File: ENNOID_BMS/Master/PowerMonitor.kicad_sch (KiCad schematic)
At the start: 103 parts, among them J15 Charge +, U1 AMC1301 or AMC1302, U10 SN6501DBV, U12 AMC1301, U13 AMC1301, U15A OPA2197IDR, U15B OPA2197IDR, U15C OPA2197IDR, U16 ISL28022, U3 TPS76350, U4 SN6501DBV, U5 SFH617A-2X009T, U6 TPS76350

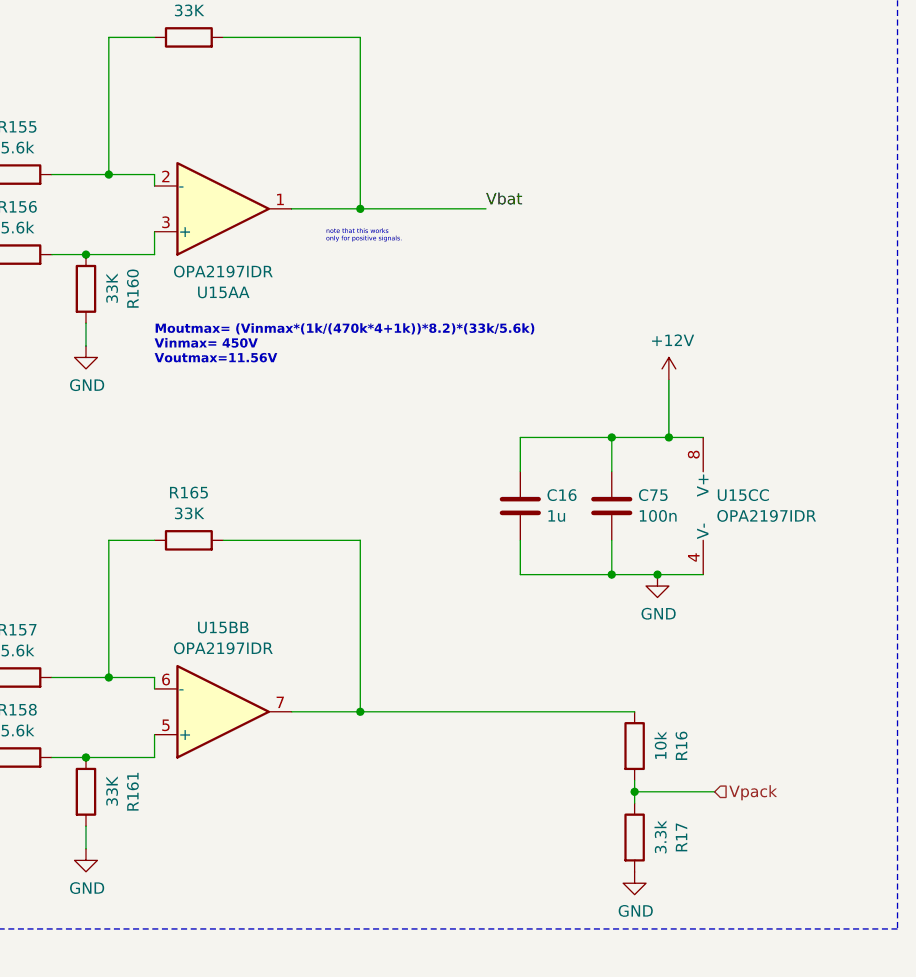
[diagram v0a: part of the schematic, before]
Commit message: ENNOID BMS PCBs completed
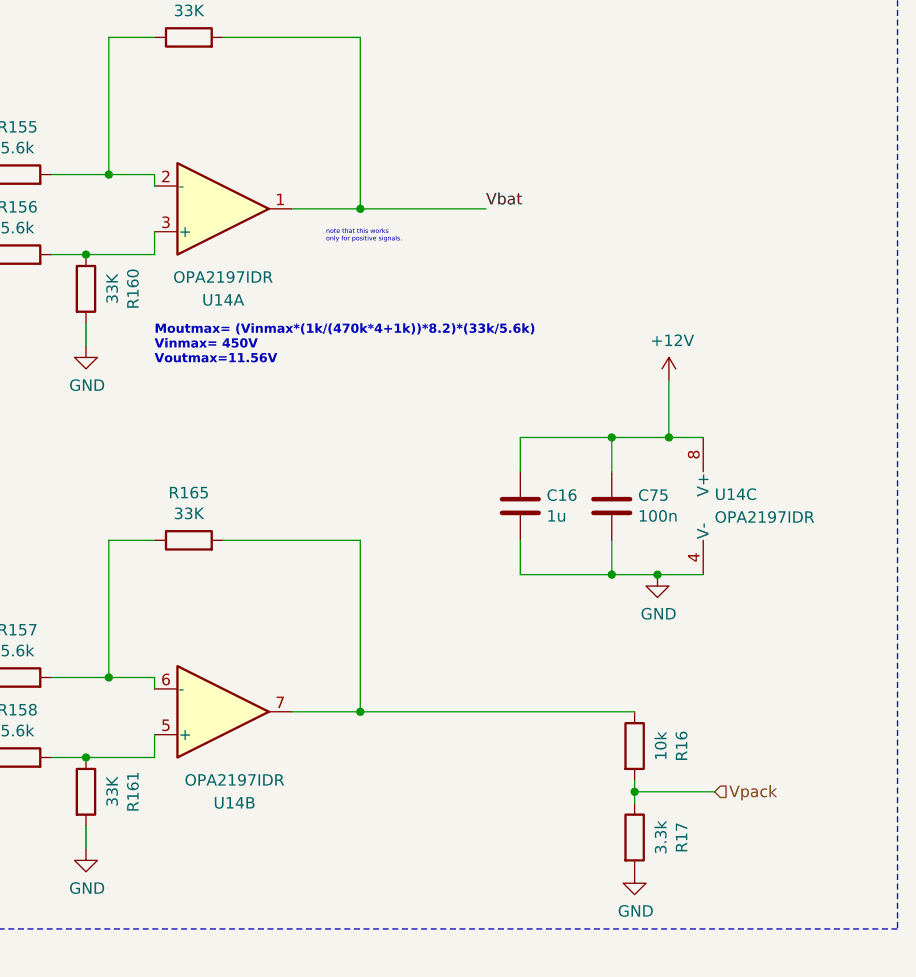
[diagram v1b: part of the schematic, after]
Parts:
- removed U15A, U15B, U15C: OPA2197IDR, Housings_SOIC:SOIC-8_3.9x4.9mm_Pitch1.27mm, symbol Amplifier_Operational:OPA2376xxD
- added U14: OPA2197IDR, Package_SO:SOIC-8_3.9x4.9mm_P1.27mm, symbol Amplifier_Operational:OPA2197xD
- D14, D15, D17, D18: footprint Diodes_SMD:D_SOD-123 -> Diode_SMD:D_SOD-123
- U1, U12, U13: footprint Housings_SOIC:SSO-8_6.8x5.9mm_Pitch1.27mm_Clearance8mm -> ENNOID:SSO-8_6.8x5.9mm_Pitch1.27mm_Clearance8mm
- U16: footprint Housings_SSOP:MSOP-10_3x3mm_Pitch0.5mm -> Package_SO:MSOP-10_3x3mm_P0.5mm
- U5: footprint Housings_DIP:SMDIP-4_W9.53mm_Clearance8mm -> Package_DIP:SMDIP-4_W9.53mm_Clearance8mm
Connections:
- net +12V: now also U14.8 (V+)
- net GND: now also U14.4 (V-)
- net Vbat: now also U14.1
- net at R156.2, R160.1: now also U14.3 (+)
- net at R155.2, R164.1: now also U14.2 (-)
- net at R157.2, R165.1: now also U14.6 (-)
- net at R158.2, R161.1: now also U14.5 (+)
- net at R16.1, R165.2: now also U14.7
